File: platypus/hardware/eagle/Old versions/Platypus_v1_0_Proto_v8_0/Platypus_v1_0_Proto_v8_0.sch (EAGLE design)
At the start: 28 parts, among them J1 EDISON_CONNECTOR_FULLMOUNTING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, U1 MPU-9150, U2 TXB0108, U3 MAX17043, X3 Power TP, X4 I2C TP, X5 Display TP

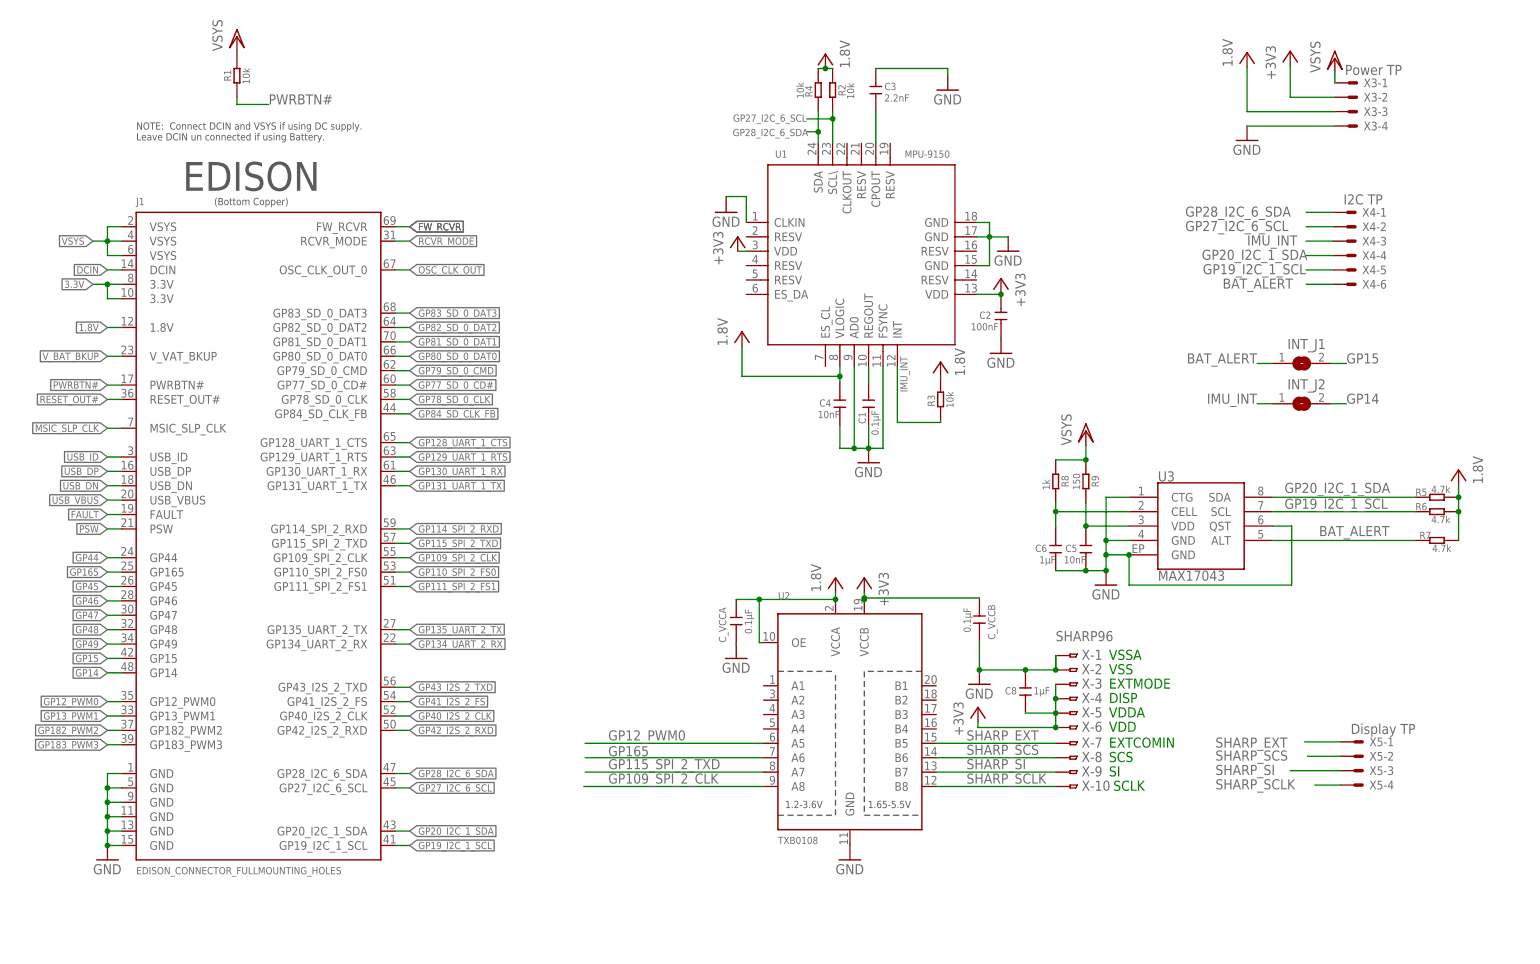
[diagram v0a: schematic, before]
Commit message: updated platypus hardware folder
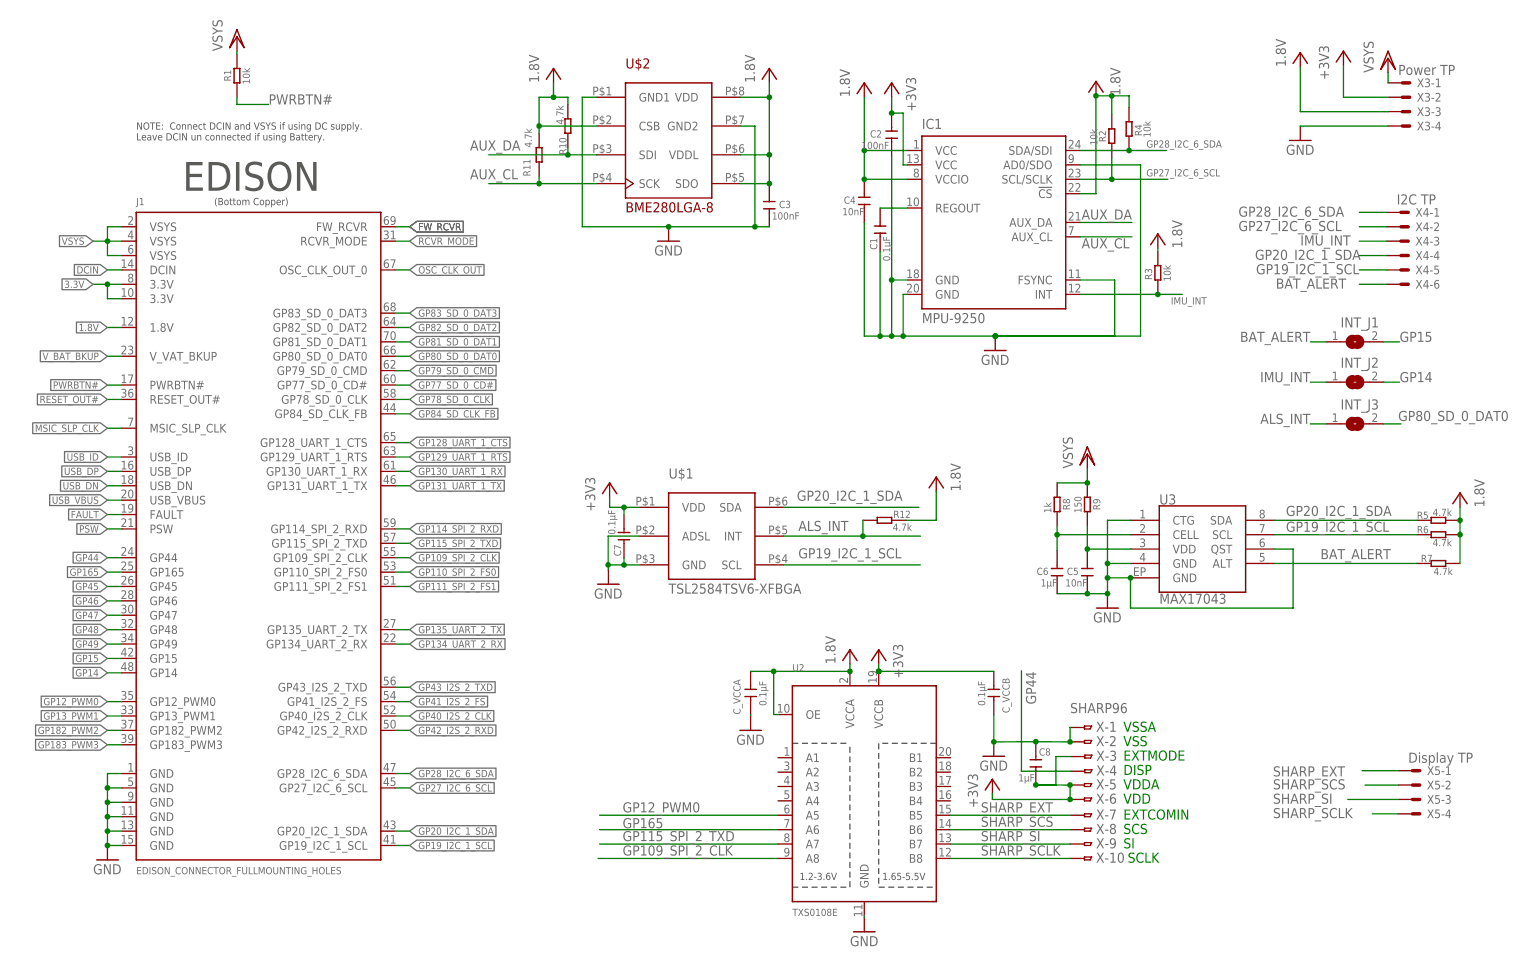
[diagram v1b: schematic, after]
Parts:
- removed U1: MPU-9150, template:MPU-9150
- added C7: 0.1µF, Discrete:C-0603
- added IC1: MPU-9250, invensense:MPU-9250
- added INT_J3: (no value), jumper:SJ
- added R10, R11, R12: 4.7k, Discrete:R-0603
- added U$1: TSL2584TSV6-XFBGA, TSL2584TSV:TSL2584TSV6-XFBGA
- added U$2: BME280LGA-8, BME280:BME280LGA-8
- C3: value 2.2nF -> 100nF
- U2: value TXB0108 -> TXS0108E
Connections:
- removed net N$2: C3.2, U1.CPOUT
- new net ALS_INT: INT_J3.1, R12.1, U$1.INT
- new net AUX_CL: IC1.AUX_CL, R11.1, U$2.SCK
- new net AUX_DA: IC1.AUX_DA, R10.1, U$2.SDI
- net 1.8V: now also C3.2, IC1.!CS, IC1.VCC@1, IC1.VCCIO, R10.2, R11.2, R12.2, U$2.CSB, U$2.SDO, U$2.VDD, U$2.VDDL; no longer U1.VLOGIC
- net 3.3V: now also C7.2, IC1.VCC@2, U$1.VDD; no longer U1.VDD, U1.VDD@1, X-4.1
- net GND: now also C7.1, IC1.AD0/SDO, IC1.FSYNC, IC1.GND@1, IC1.GND@2, U$1.ADSL, U$1.GND, U$2.GND1, U$2.GND2; no longer U1.AD0, U1.CLKIN, U1.FSYNC, U1.GND, U1.GND@1, U1.GND@2
- net GP19_I2C_1_SCL: now also U$1.SCL
- net GP20_I2C_1_SDA: now also U$1.SDA
- net GP27_I2C_6_SCL: now also IC1.SCL/SCLK; no longer U1.SCL\
- net GP28_I2C_6_SDA: now also IC1.SDA/SDI; no longer U1.SDA
- net GP44: now also X-4.1
- net GP80_SD_0_DAT0: now also INT_J3.2
- net IMU_INT: now also IC1.INT; no longer U1.INT
- net N$5: now also IC1.REGOUT; no longer U1.REGOUT
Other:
- moved on the sheet: C1, C2, C3, C4, C5, C6, C8, C_VCCA, C_VCCB, INT_J1, INT_J2, R2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
